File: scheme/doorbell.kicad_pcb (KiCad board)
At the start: 2 copper layers, 50 x 25 mm, 13 parts

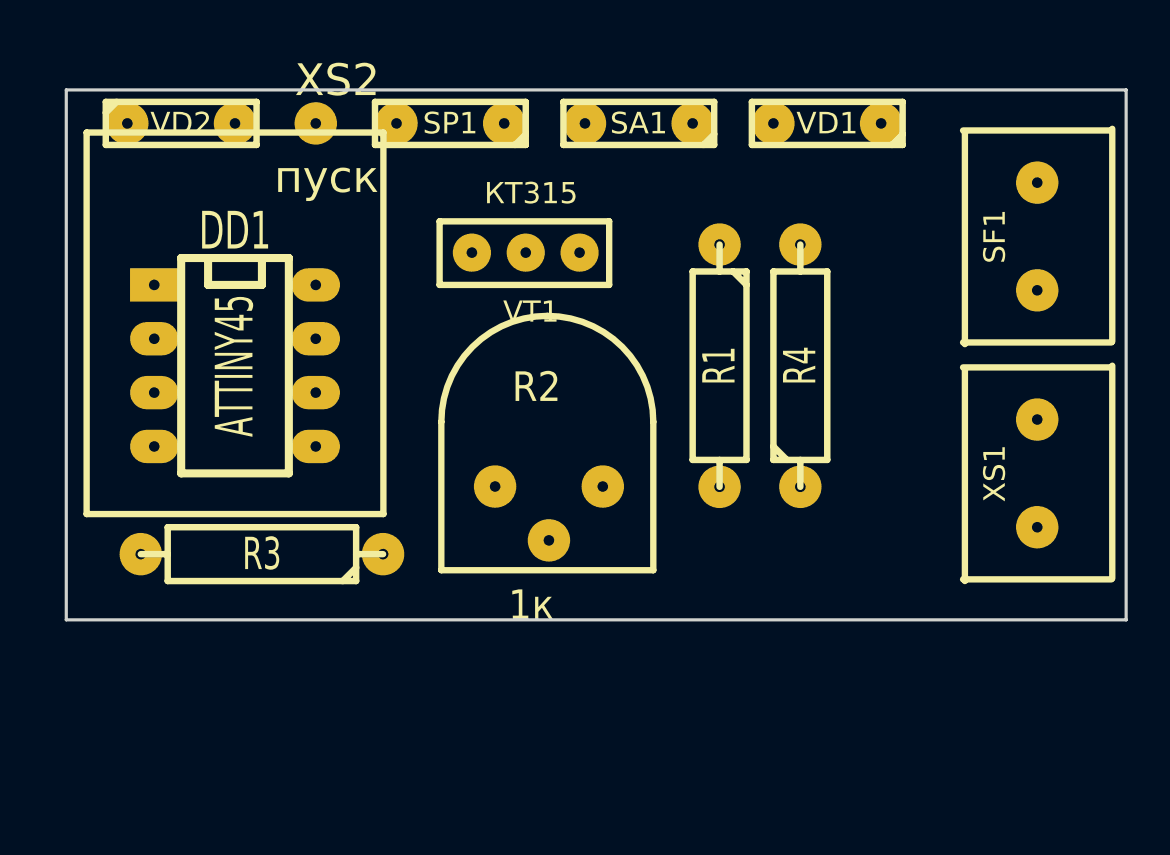
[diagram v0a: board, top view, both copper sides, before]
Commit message: small changes
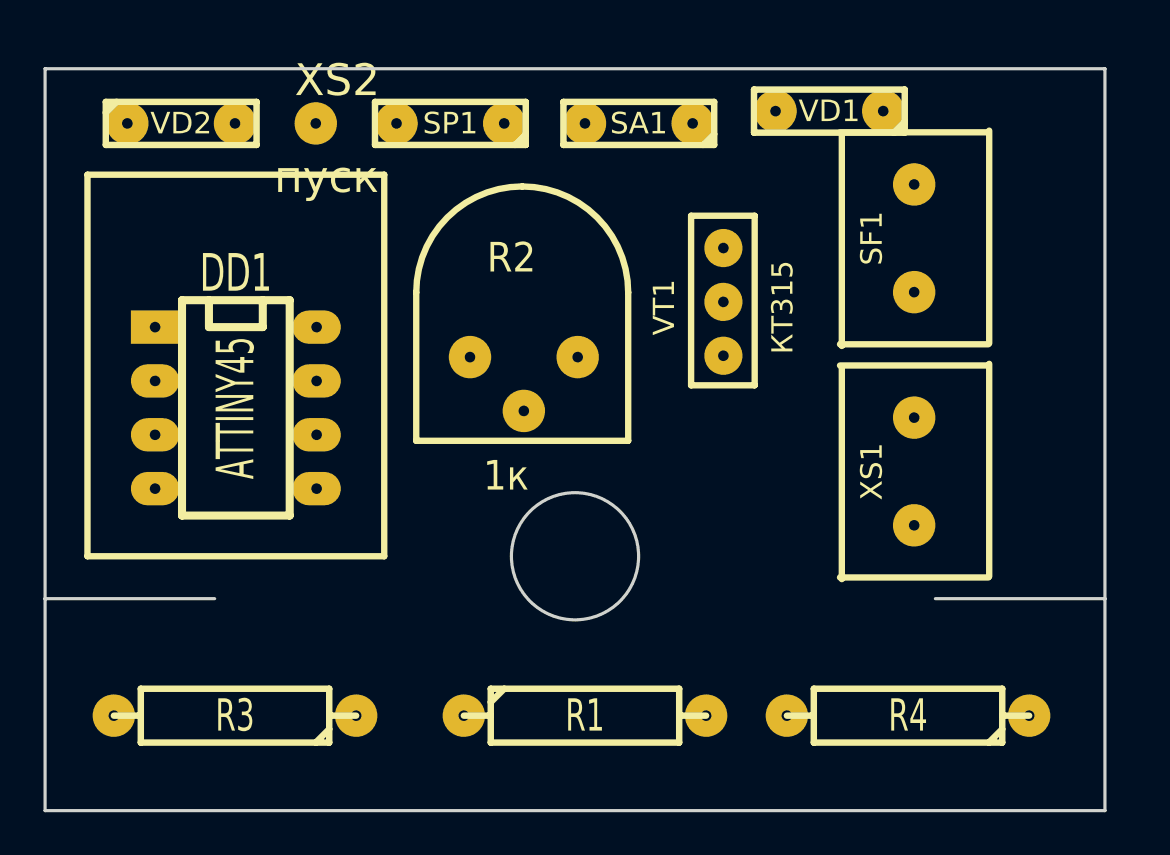
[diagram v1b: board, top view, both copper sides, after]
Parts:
- moved R1 17.7 mm to (77.5, 96.5), turned to 0 degrees
- moved R4 17.3 mm to (92.7, 96.5), turned to 180 degrees
- moved VT1 9.61 mm to (84.0, 77.0), turned to 270 degrees
- moved R3 7.73 mm to (61.0, 96.5)
- moved R2 6.22 mm to (74.0, 80.0)
- moved XS1 5.81 mm to (93.0, 85.0)
- moved SF1 5.81 mm to (93.0, 74.0)
- moved DD1 1.99 mm to (61.0, 82.0)
- moved VD1 0.59 mm to (89.0, 68.0)
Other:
- board size 50 x 25 mm -> 50 x 35 mm

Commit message: next step
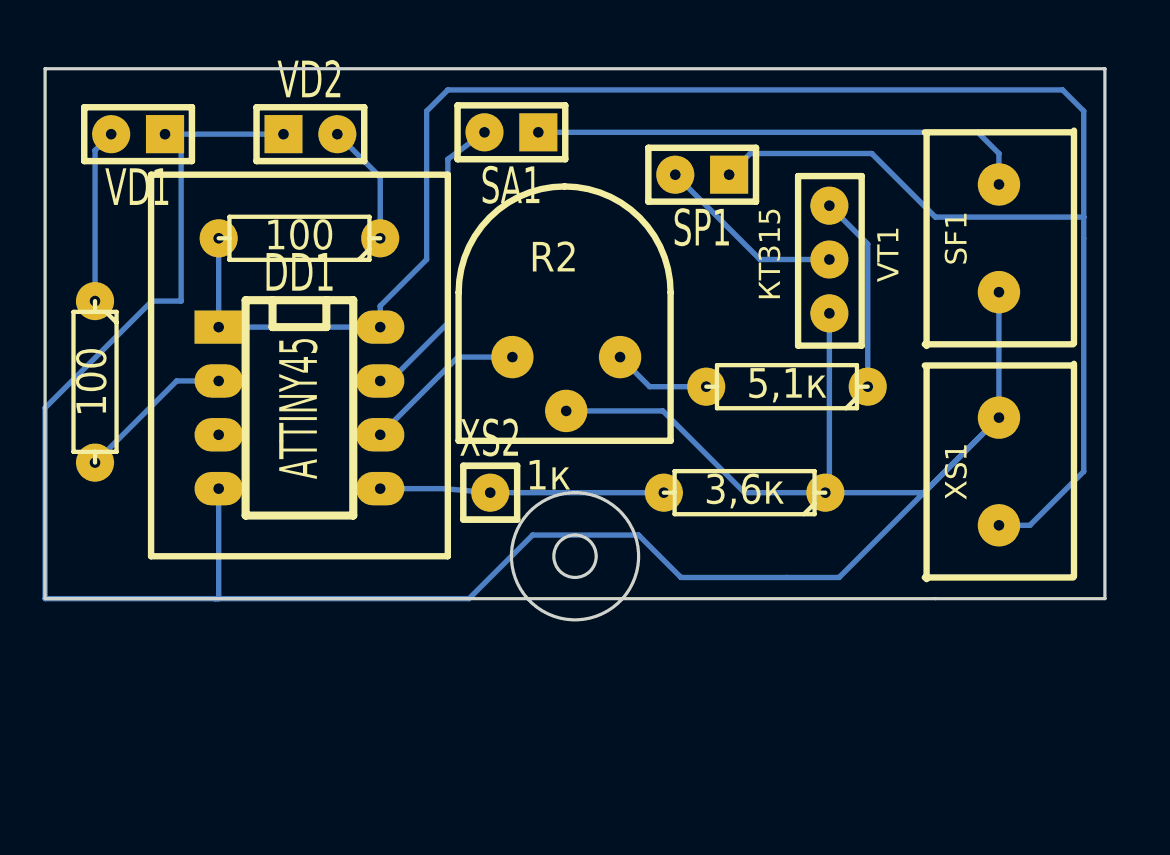
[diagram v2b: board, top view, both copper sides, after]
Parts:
- added R5: 3,6к, R3, F.Cu at (85.0, 86.0)
- R1, R3, R4: footprint R4-5 -> R3
- SA1, SP1: footprint C2 -> SIL-2
- VD1: value LED -> красный; footprint C2 -> SIL-2
- VD2: value LED -> зеленый; footprint C2 -> SIL-2
- XS2: footprint 1pinsmall -> SIL-1
- moved R4 36.5 mm to (64.0, 74.0)
- moved VD1 32.6 mm to (56.4, 69.1)
- moved XS2 19.3 mm to (73.0, 86.0)
- moved R1 18.2 mm to (87.0, 81.0), turned to 180 degrees
- moved R3 17.1 mm to (54.4, 80.8), turned to 270 degrees
- moved SP1 12.1 mm to (83.0, 71.0)
- moved VD2 6.12 mm to (64.5, 69.1)
- moved SA1 6.02 mm to (74.0, 69.0)
- moved VT1 5.39 mm to (89.0, 75.0), turned to 90 degrees
- moved SF1 4.00 mm to (97.0, 74.0)
- moved XS1 4.00 mm to (97.0, 85.0)
- moved DD1 3.00 mm to (64.0, 82.0)
- moved R2 2.00 mm to (76.0, 80.0)
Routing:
- net GND: track 0.00 -> 124.8 mm
- net V+: track 0.00 -> 95.2 mm
- net N-000009: track 0.00 -> 23.6 mm
- net N-0000011: track 0.00 -> 14.2 mm
- net N-0000010: track 0.00 -> 13.4 mm
- net N-000004: track 0.00 -> 9.29 mm
- net N-000003: track 0.00 -> 8.93 mm
- net N-000007: track 0.00 -> 8.19 mm
- net N-000005: track 0.00 -> 7.75 mm
- net N-000002: track 0.00 -> 7.43 mm
- net N-0000012: track 0.00 -> 5.75 mm
- net N-000001: track 0.00 -> 4.64 mm
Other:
- board size 50 x 35 mm -> 50 x 26 mm

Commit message: small changes
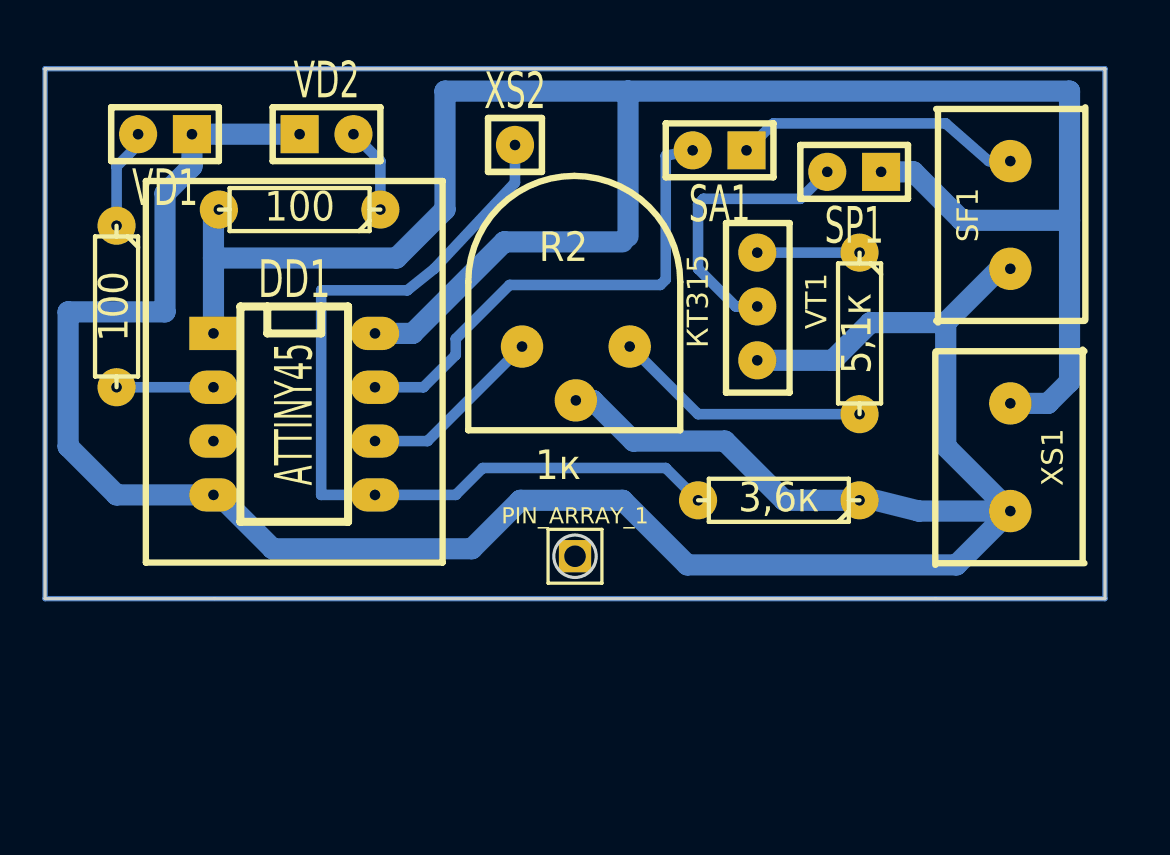
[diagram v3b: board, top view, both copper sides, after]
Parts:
- added PIN_ARRAY_1: Val**, PIN_ARRAY_1, F.Cu at (77.0, 89.0)
- moved XS2 16.4 mm to (74.2, 69.6)
- moved SA1 9.86 mm to (83.8, 69.8)
- moved SP1 7.17 mm to (90.2, 70.9)
- moved R1 4.25 mm to (90.4, 78.5), turned to 270 degrees
- moved VT1 4.06 mm to (85.6, 77.2)
- moved R3 3.70 mm to (55.4, 77.2)
- moved R5 1.65 mm to (86.6, 86.4)
- moved R4 1.36 mm to (64.0, 72.6)
- moved VD1 1.27 mm to (57.7, 69.1)
- moved SF1 1.23 mm to (97.5, 72.9)
- moved XS1 0.86 mm to (97.5, 84.3), turned to 270 degrees
- moved VD2 0.76 mm to (65.3, 69.1)
- moved R2 0.67 mm to (76.5, 79.5)
- moved DD1 0.38 mm to (63.8, 82.3)
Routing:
- net (no net): track 0.00 -> 150.0 mm
- net N-0000010: track 13.4 -> 41.6 mm
- net N-000009: track 23.6 -> 14.0 mm
- net N-0000011: track 14.2 -> 23.4 mm
- net N-000001: track 4.64 -> 12.2 mm
- net V+: track 95.2 -> 100.3 mm
- net N-000004: track 9.29 -> 4.83 mm
- net N-000003: track 8.93 -> 13.3 mm
- net GND: track 124.8 -> 121.0 mm
- net N-000007: track 8.19 -> 4.74 mm
- net N-000002: track 7.43 -> 4.57 mm
- net N-0000012: track 5.75 -> 4.08 mm
- net N-000005: track 7.75 -> 8.78 mm
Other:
- board size 50 x 26 mm -> 50 x 25 mm
